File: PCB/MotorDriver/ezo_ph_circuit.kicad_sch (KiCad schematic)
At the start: 4 parts, among them U3 EZO, U4 Molex_SMA

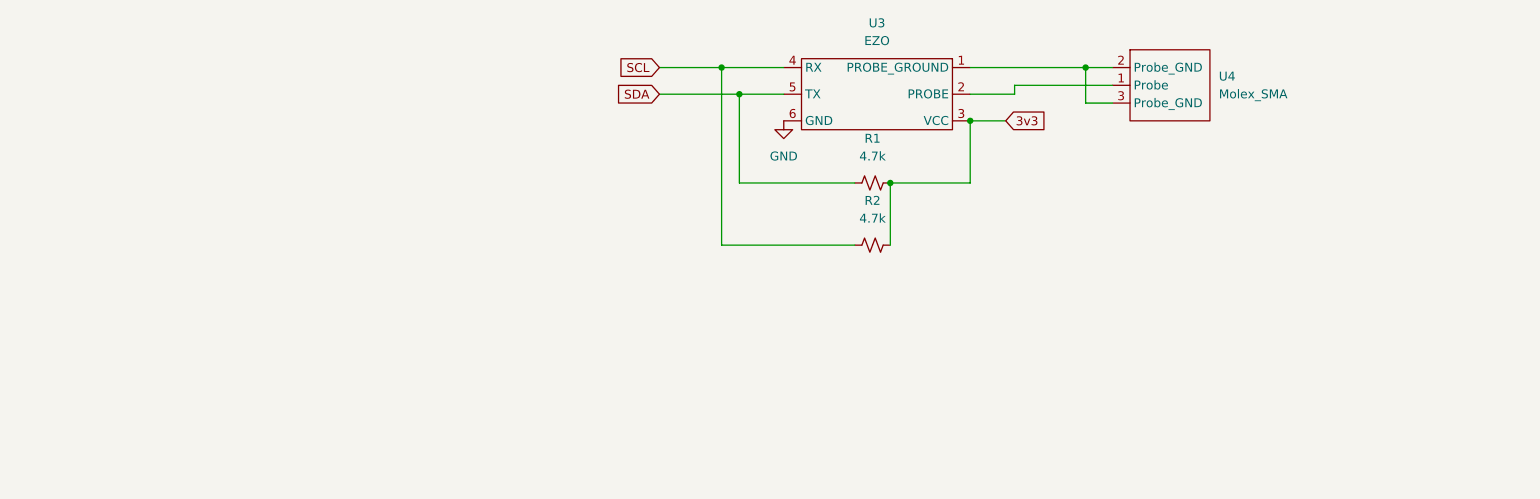
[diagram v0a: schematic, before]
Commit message: Add wifi and DB
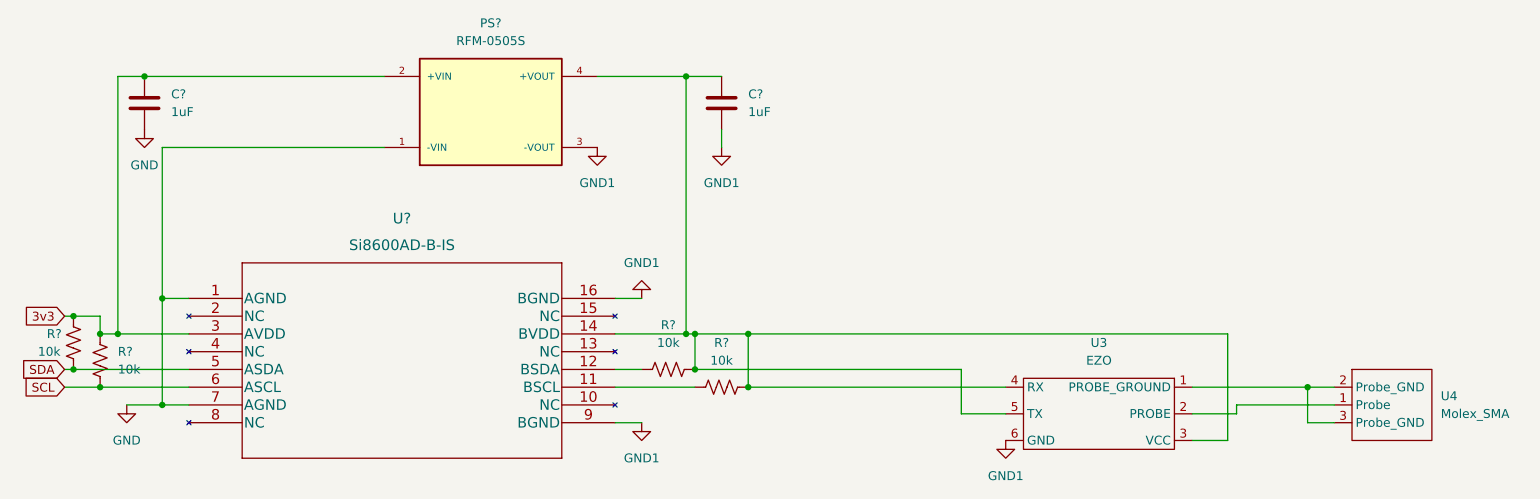
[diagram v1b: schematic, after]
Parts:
- removed R1, R2: 4.7k, Resistor_THT:R_Axial_DIN0207_L6.3mm_D2.5mm_P10.16mm_Horizontal, symbol Device:R_Small_US
- added C? (x2): 1uF, symbol Device:C
- added PS?: RFM-0505S, SnapEDA Library:CONV_RFM-0505S, symbol RFM-0505S:RFM-0505S
- added R? (x4): 10k, symbol Device:R_US
- added U?: Si8600AD-B-IS, SOIC-16W_SIL, symbol SI8600AD-B-IS:Si8600AD-B-IS
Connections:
- net 3v3: now also C?.1, PS?.2 (+VIN), R?.1, R?.2, U?.3 (AVDD); no longer U3.3 (VCC)
- net GND: now also C?.2, PS?.1 (-VIN), U?.1 (AGND), U?.7 (AGND); no longer U3.6 (GND)
- net SCL: now also R?.1, U?.6 (ASCL); no longer U3.4 (RX)
- net SDA: now also R?.2, U?.5 (ASDA); no longer U3.5 (TX)
- new net: C?.1, PS?.4 (+VOUT), R?.1, R?.1, U3.3 (VCC), U3.4 (RX), U3.5 (TX), U?.14 (BVDD)
- new net: R?.2, U?.12 (BSDA)
- new net: R?.2, U?.11 (BSCL)
- new net GND1: C?.2, PS?.3 (-VOUT), U3.6 (GND), U?.16 (BGND), U?.9 (BGND)
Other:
- moved on the sheet: U3, U4
